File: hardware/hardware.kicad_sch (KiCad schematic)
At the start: 21 parts, among them J1 5V, J2 GND, J3 RESET, J4 MISO, J5 MOSI, J6 SCK, J7 CS, J8 VIN, J9 VOUT, U1 MAX7456EUI+, Y1 Resonator

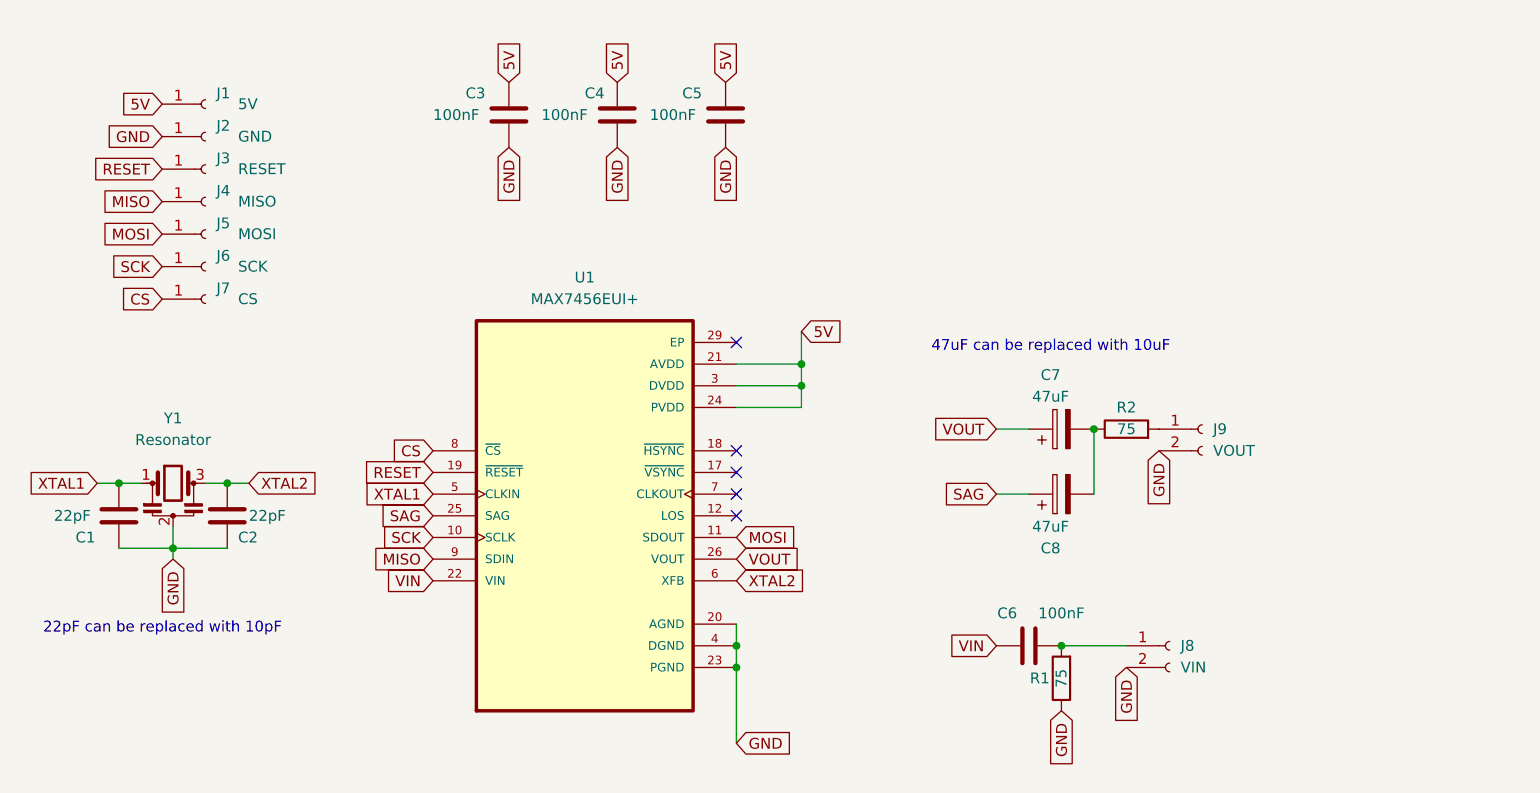
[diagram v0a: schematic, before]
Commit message: redesign
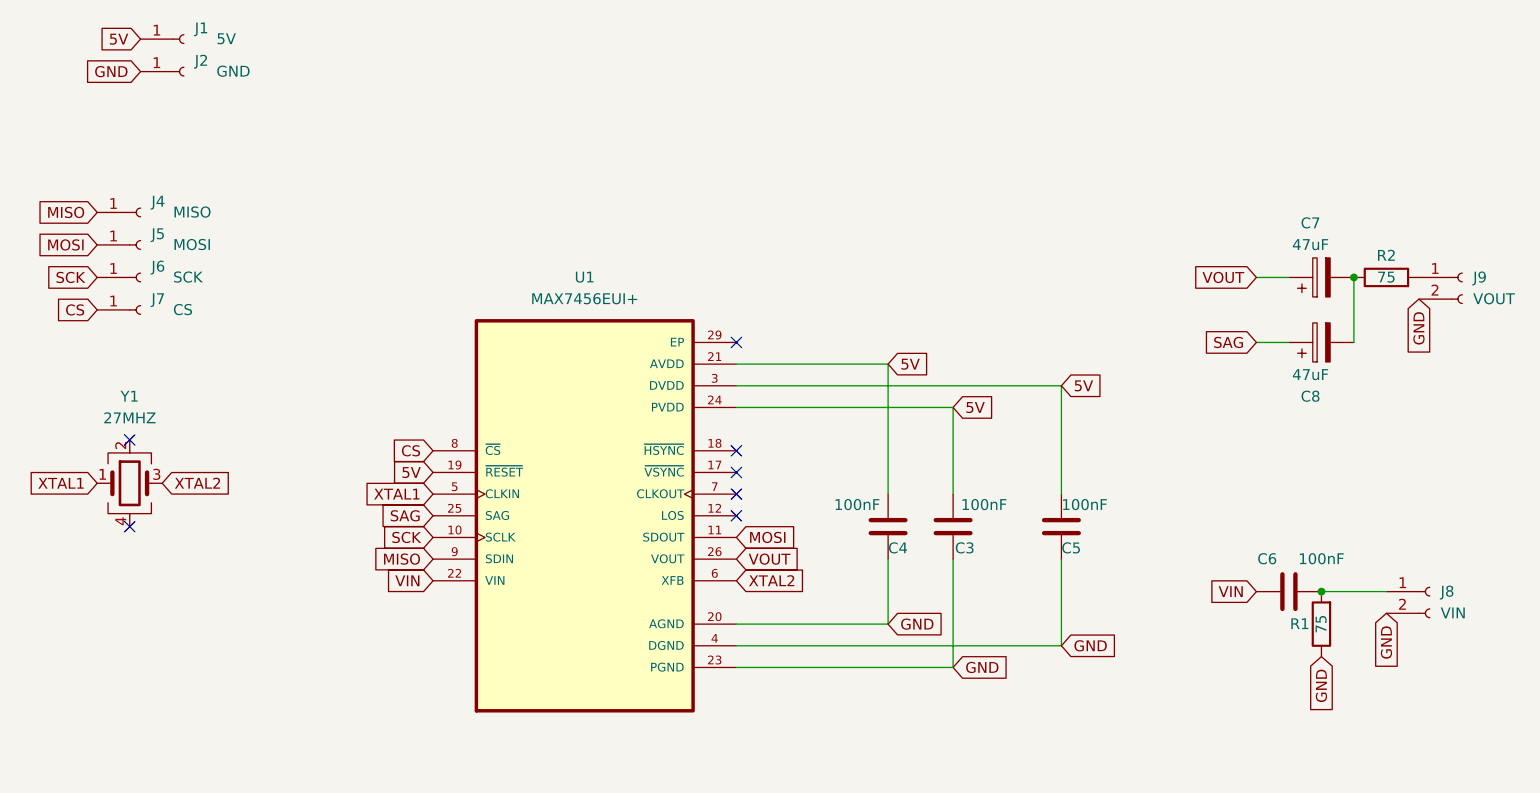
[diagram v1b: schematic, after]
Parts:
- removed C1, C2: 22pF, Capacitor_SMD:C_0805_2012Metric_Pad1.18x1.45mm_HandSolder, symbol Device:C
- removed J3: RESET, Connector_PinHeader_2.54mm:PinHeader_1x01_P2.54mm_Vertical, symbol Connector:Conn_01x01_Female
- removed Y1: Resonator, Crystal:Crystal_SMD_3225-4Pin_3.2x2.5mm_HandSoldering, symbol Device:Resonator
- added Y1: 27MHZ, Crystal:Crystal_SMD_3225-4Pin_3.2x2.5mm_HandSoldering, symbol Device:Crystal_GND24
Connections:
- net RESET is gone; now on net 5V: U1.19 (~{RESET})
- net 5V: now also C3.2; no longer C3.1
- net GND: now also C3.1; no longer C3.2
- net XTAL1: now also Y1.1
- net XTAL2: now also Y1.3
- no-connect marks 5 -> 7
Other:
- note removed: "22pF can be replaced with 10pF"
- note removed: "47uF can be replaced with 10uF"
- moved on the sheet: C3, C4, C5, C6, C7, C8, J1, J2, J4, J5, J6, J7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
